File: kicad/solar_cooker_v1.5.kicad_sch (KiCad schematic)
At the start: 28 parts, among them J1 Pt100, J10 SSQ-108-01-G-S, J11 SSQ-108-01-G-S, J12 SSQ-108-01-G-S, J13 SSQ-118-01-G-D, J14 SSQ-108-01-G-S, J15 SSQ-108-01-G-S, J16 SSQ-110-01-G-S, J4 Pt100, J6 GPS, J7 Pt100, J8 display, J9 SSQ-109-01-G-S, U2 microSD, U3 clock_module, U3 pyranometer, U5 anemometer, U6 BME680, U9 AM2315C

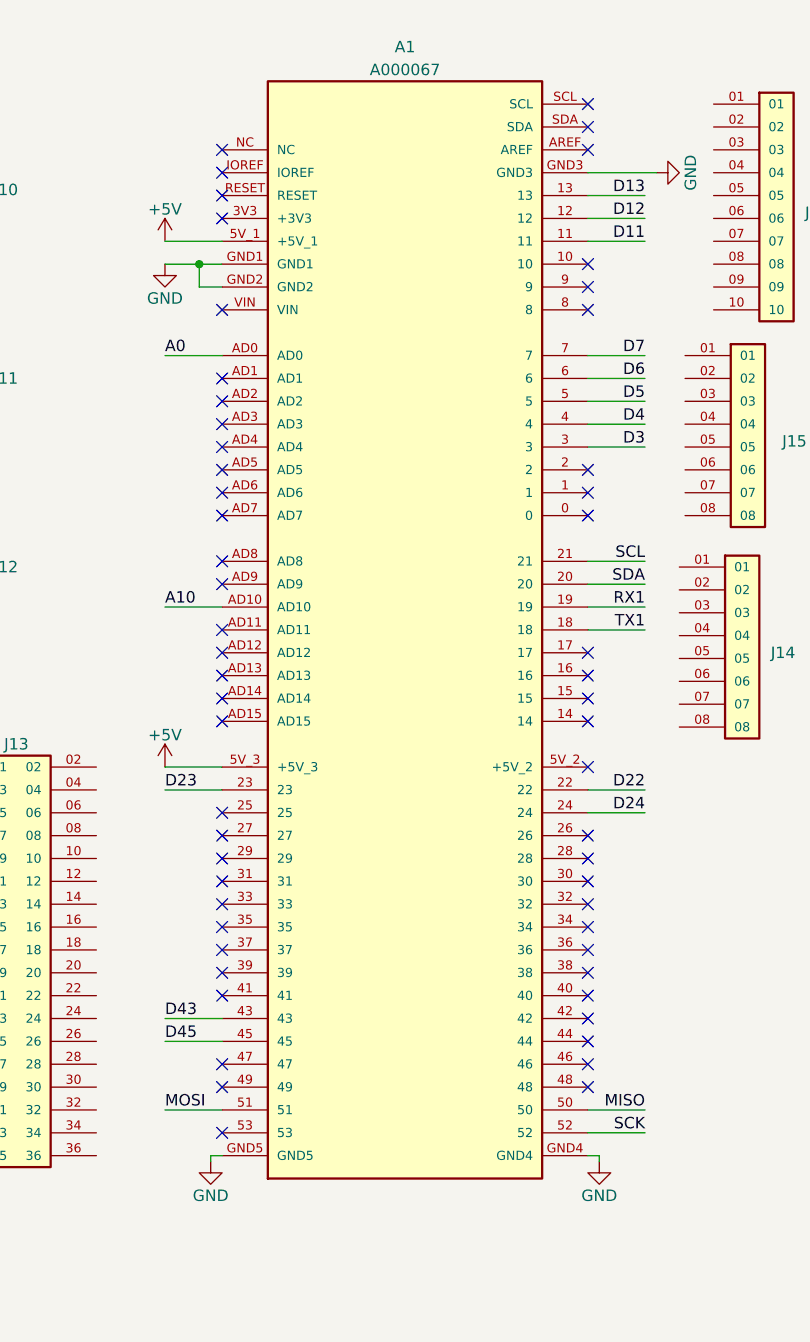
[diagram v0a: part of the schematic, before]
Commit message: order v2
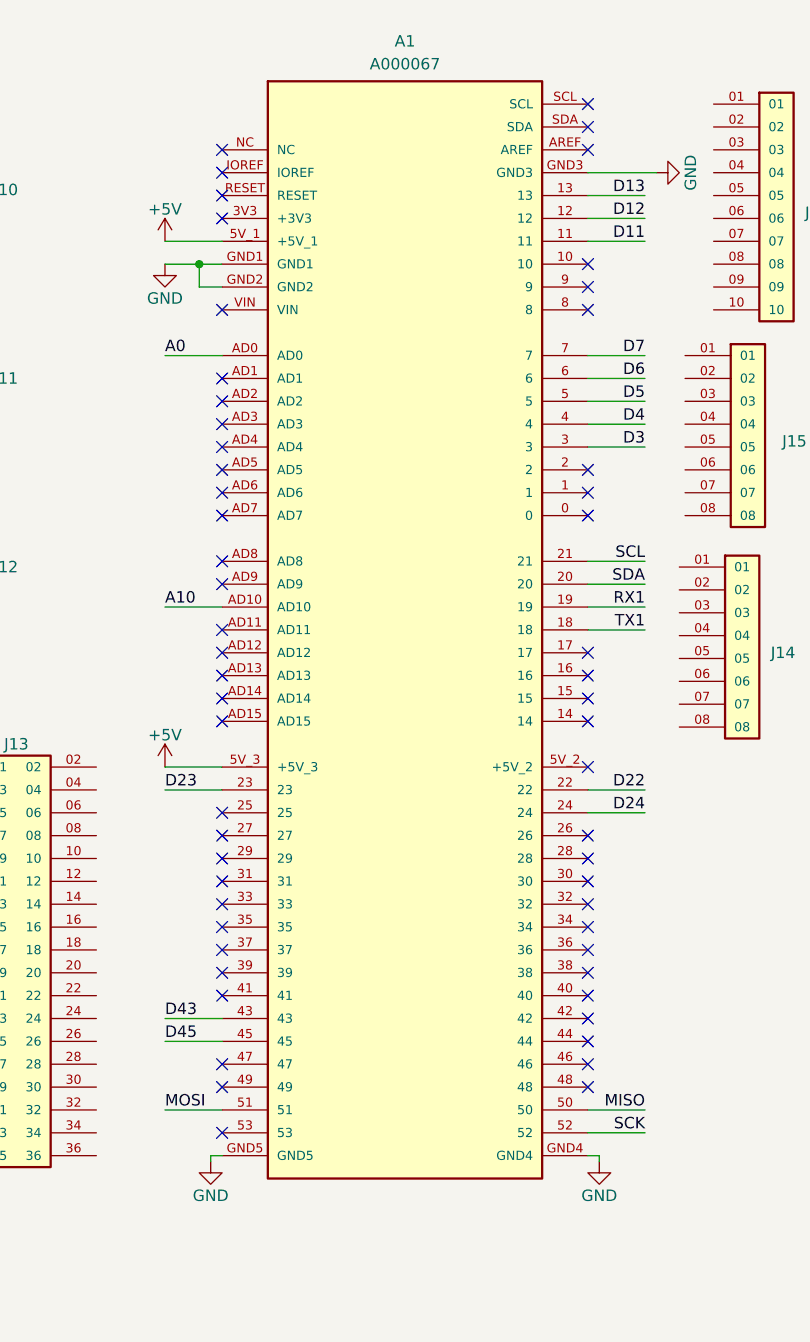
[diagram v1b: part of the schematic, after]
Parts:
- D? (x2): footprint (none) -> LED_SMD:LED_1206_3216Metric_Pad1.42x1.75mm_HandSolder
- J1, J4, J7: footprint custom_components:Pt100 -> custom_components:PT100
- J6: footprint (none) -> custom_components:GPS
- J8: footprint (none) -> custom_components:display
- PS1: footprint CONV_TBA_1-0519 -> TBA_1-0519:CONV_TBA_1-0519; MANUFACTURER Traco Power -> (none); MAXIMUM_PACKAGE_HEIGHT 10.15mm -> (none); PARTREV April 19, 2021 -> (none); STANDARD Manufacturer Recommendations -> (none)
- R1, R? (x2): footprint (none) -> Resistor_SMD:R_1206_3216Metric_Pad1.30x1.75mm_HandSolder
- U2: footprint (none) -> custom_components:microSD
- U3, U9: footprint (none) -> custom_components:screw_terminal_4pin
- U3: footprint (none) -> custom_components:clock_module
- U5: footprint (none) -> custom_components:screw_terminal_3pin
- U6: footprint (none) -> custom_components:BME680
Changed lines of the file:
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@@
     (stroke (width 0) (type default) (color 255 0 0 1))
+  )
+  (wire (pts (xy 208.915 57.785) (xy 215.265 57.785))
+    (stroke (width 0) (type default))
   )
   (wire (pts (xy 153.035 46.99) (xy 153.035 49.53))
@@
     (stroke (width 0) (type default))
   )
-  (wire (pts (xy 208.915 57.785) (xy 215.265 57.785))
-    (stroke (width 0) (type default))
-  )
   (wire (pts (xy 38.735 123.825) (xy 44.45 123.825))
     (stroke (width 0) (type default) (color 1 1 1 1))
@@
     (effects (font (size 1.27 1.27)) (justify left bottom))
   )
+  (label "A0" (at 208.915 57.785 0) (fields_autoplaced)
+    (effects (font (size 1.27 1.27)) (justify left bottom))
+  )
   (label "SCK" (at 62.484 161.925 180) (fields_autoplaced)
     (effects (font (size 1.27 1.27)) (justify right bottom))
@@
     (effects (font (size 1.27 1.27)) (justify left bottom))
   )
-  (label "A0" (at 208.915 57.785 0) (fields_autoplaced)
-    (effects (font (size 1.27 1.27)) (justify left bottom))
-  )
   (label "D12" (at 96.393 154.178 180) (fields_autoplaced)
     (effects (font (size 1.27 1.27)) (justify right bottom))
@@
       (effects (font (size 1.27 1.27)))
     )
-    (property "Footprint" "" (at 112.395 93.98 0)
+    (property "Footprint" "custom_components:display" (at 112.395 93.98 0)
       (effects (font (size 1.27 1.27)) hide)
     )
@@
       (effects (font (size 1.27 1.27)))
     )
-    (property "Footprint" "" (at 49.53 117.475 0)
+    (property "Footprint" "custom_components:screw_terminal_4pin" (at 49.53 117.475 0)
       (effects (font (size 1.27 1.27)) hide)
     )
@@
       (effects (font (size 1.27 1.27)) (justify left))
     )
-    (property "Footprint" "" (at 104.775 39.37 0)
+    (property "Footprint" "Resistor_SMD:R_1206_3216Metric_Pad1.30x1.75mm_HandSolder" (at 104.775 39.37 0)
       (effects (font (size 1.27 1.27)) hide)
     )
@@
       (effects (font (size 1.27 1.27)))
     )
-    (property "Footprint" "" (at 153.035 35.56 0)
+    (property "Footprint" "LED_SMD:LED_1206_3216Metric_Pad1.42x1.75mm_HandSolder" (at 153.035 35.56 0)
       (effects (font (size 1.27 1.27)) hide)
     )
@@
       (effects (font (size 1.27 1.27)) (justify left))
     )
-    (property "Footprint" "" (at 72.39 94.615 0)
+    (property "Footprint" "Resistor_SMD:R_1206_3216Metric_Pad1.30x1.75mm_HandSolder" (at 72.39 94.615 0)
       (effects (font (size 1.27 1.27)) hide)
     )
@@
       (effects (font (size 1.27 1.27)))
     )
-    (property "Footprint" "" (at 52.07 27.94 0)
+    (property "Footprint" "custom_components:microSD" (at 52.07 27.94 0)
       (effects (font (size 1.27 1.27)) hide)
     )
@@
       (effects (font (size 1.27 1.27)) (justify left))
     )
-    (property "Footprint" "" (at 153.035 44.45 0)
+    (property "Footprint" "Resistor_SMD:R_1206_3216Metric_Pad1.30x1.75mm_HandSolder" (at 153.035 44.45 0)
       (effects (font (size 1.27 1.27)) hide)
     )
@@
       (effects (font (size 1.27 1.27)))
     )
-    (property "Footprint" "custom_components:Pt100" (at 73.406 149.098 0)
+    (property "Footprint" "custom_components:PT100" (at 73.406 149.098 0)
       (effects (font (size 1.27 1.27)) hide)
     )
@@
       (effects (font (size 1.27 1.27)))
     )
-    (property "Footprint" "" (at 137.16 35.56 0)
+    (property "Footprint" "LED_SMD:LED_1206_3216Metric_Pad1.42x1.75mm_HandSolder" (at 137.16 35.56 0)
       (effects (font (size 1.27 1.27)) hide)
     )
@@
       (effects (font (size 1.27 1.27)))
     )
-    (property "Footprint" "" (at 85.09 60.325 0)
+    (property "Footprint" "custom_components:screw_terminal_4pin" (at 85.09 60.325 0)
       (effects (font (size 1.27 1.27)) hide)
     )
@@
       (effects (font (size 1.27 1.27)))
     )
-    (property "Footprint" "custom_components:Pt100" (at 39.497 149.225 0)
+    (property "Footprint" "custom_components:PT100" (at 39.497 149.225 0)
       (effects (font (size 1.27 1.27)) hide)
     )
@@
       (effects (font (size 1.27 1.27)))
     )
-    (property "Footprint" "custom_components:Pt100" (at 106.426 149.098 0)
+    (property "Footprint" "custom_components:PT100" (at 106.426 149.098 0)
       (effects (font (size 1.27 1.27)) hide)
     )
@@
       (effects (font (size 1.27 1.27)) (justify left))
     )
-    (property "Footprint" "" (at 137.16 44.45 0)
+    (property "Footprint" "Resistor_SMD:R_1206_3216Metric_Pad1.30x1.75mm_HandSolder" (at 137.16 44.45 0)
       (effects (font (size 1.27 1.27)) hide)
     )
@@
       (effects (font (size 1.27 1.27)))
     )
-    (property "Footprint" "" (at 53.34 98.425 0)
+    (property "Footprint" "custom_components:screw_terminal_3pin" (at 53.34 98.425 0)
       (effects (font (size 1.27 1.27)) hide)
     )
@@
   (symbol (lib_id "A000067:A000067") (at 235.585 88.265 0) (unit 1)
     (in_bom no) (on_board yes) (dnp no) (fields_autoplaced)
-    (property "Reference" "A1" (at 235.585 23.495 0)
-      (effects (font (size 1.27 1.27)))
-    )
-    (property "Value" "A000067" (at 235.585 26.035 0)
+    (property "Reference" "A1" (at 235.585 22.86 0)
+      (effects (font (size 1.27 1.27)))
+    )
+    (property "Value" "A000067" (at 235.585 25.4 0)
       (effects (font (size 1.27 1.27)))
     )
@@
     (pin "8")
     (pin "9")
-    (pin "AD0")
     (pin "AD1")
     (pin "AD10")
@@
     (pin "SDA")
     (pin "VIN")
+    (pin "AD0")
     (instances
       (project "solar_cooker_v1.5"
@@
       (effects (font (size 1.27 1.27)))
     )
-    (property "Footprint" "" (at 87.63 34.29 0)
+    (property "Footprint" "custom_components:BME680" (at 87.63 34.29 0)
       (effects (font (size 1.27 1.27)) hide)
     )
@@
       (effects (font (size 1.27 1.27)))
     )
-    (property "Footprint" "" (at 85.09 90.805 0)
+    (property "Footprint" "custom_components:GPS" (at 85.09 90.805 0)
       (effects (font (size 1.27 1.27)) hide)
     )
@@
       (effects (font (size 1.27 1.27)))
     )
-    (property "Footprint" "" (at 52.07 67.945 0)
+    (property "Footprint" "custom_components:clock_module" (at 52.07 67.945 0)
       (effects (font (size 1.27 1.27)) hide)
     )
@@
       (effects (font (size 1.27 1.27)))
     )
-    (property "Footprint" "CONV_TBA_1-0519" (at 124.46 69.215 0)
+    (property "Footprint" "TBA_1-0519:CONV_TBA_1-0519" (at 124.46 69.215 0)
       (effects (font (size 1.27 1.27)) (justify bottom) hide)
     )
@@
       (effects (font (size 1.27 1.27)) hide)
     )
-    (property "PARTREV" "April 19, 2021" (at 124.46 69.215 0)
-      (effects (font (size 1.27 1.27)) (justify bottom) hide)
-    )
-    (property "STANDARD" "Manufacturer Recommendations" (at 124.46 69.215 0)
-      (effects (font (size 1.27 1.27)) (justify bottom) hide)
-    )
-    (property "MAXIMUM_PACKAGE_HEIGHT" "10.15mm" (at 124.46 69.215 0)
-      (effects (font (size 1.27 1.27)) (justify bottom) hide)
-    )
-    (property "MANUFACTURER" "Traco Power" (at 124.46 69.215 0)
-      (effects (font (size 1.27 1.27)) (justify bottom) hide)
-    )
     (property "Description" "DC DC CONVERTER 9V 990MW" (at 124.46 69.215 0)
